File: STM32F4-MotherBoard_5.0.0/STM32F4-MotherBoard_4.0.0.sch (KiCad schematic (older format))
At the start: 1 part

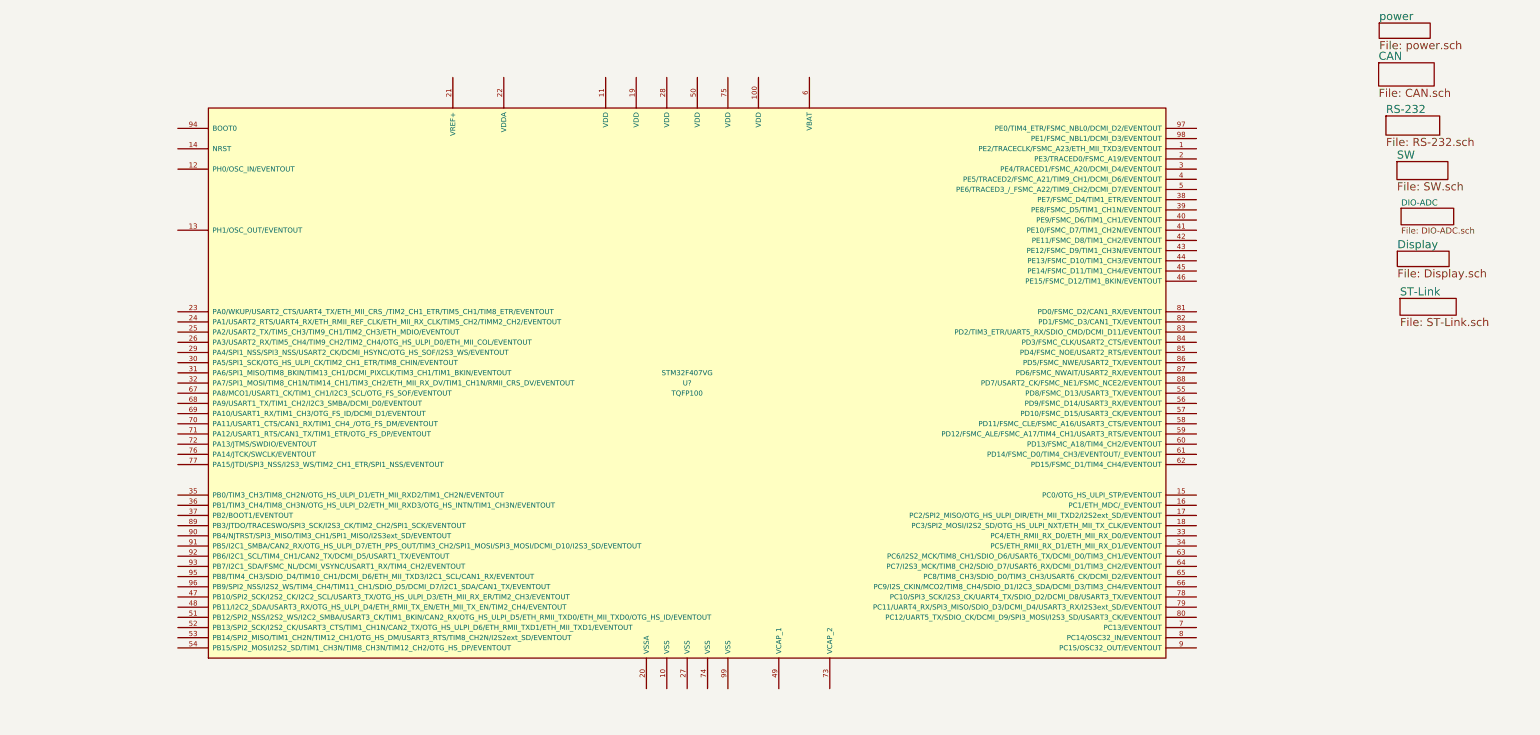
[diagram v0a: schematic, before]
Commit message: シート追加
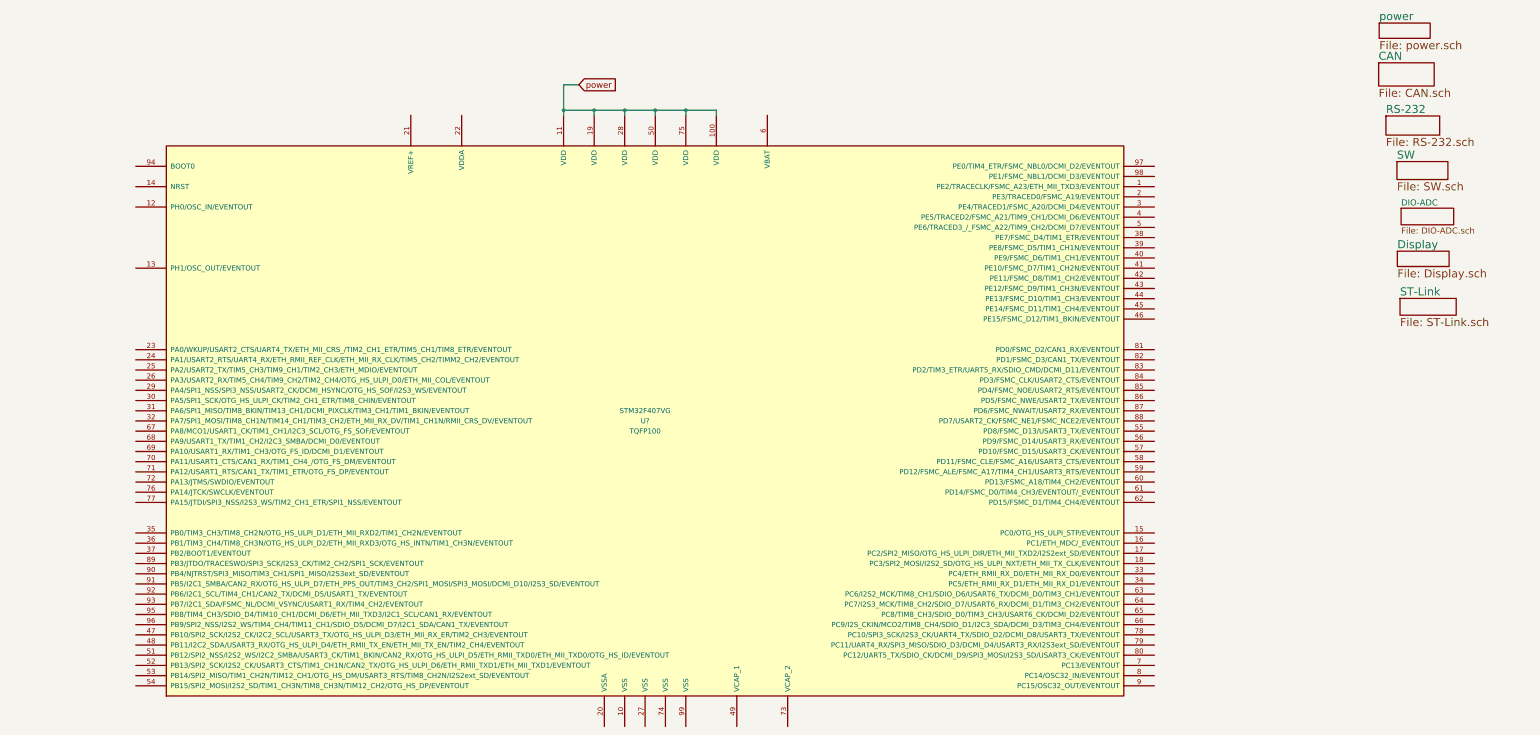
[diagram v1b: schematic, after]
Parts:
- removed U?: STM32F407VG, TQFP100, symbol STM32F407VG
- added U?: STM32F407VG, TQFP100, symbol STM32F407VG
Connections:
- new net power: U?.100 (VDD), U?.11 (VDD), U?.19 (VDD), U?.28 (VDD), U?.50 (VDD), U?.75 (VDD)
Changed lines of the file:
@@
 Comment4 ""
 $EndDescr
-$Comp
-L STM32F407VG U?
-U 1 1 589AA55C
-P 8063 5478
-F 0 "U?" H 8063 5478 50  0000 C CNN
-F 1 "STM32F407VG" H 8063 5578 50  0000 C CNN
-F 2 "TQFP100" H 8063 5378 50  0000 C CNN
-F 3 "" H 8063 5478 50  0000 C CNN
-	1    8063 5478
-	1    0    0    -1
-$EndComp
 $Sheet
 S 14857 1944 500  150
@@
 F1 "ST-Link.sch" 79
 $EndSheet
+$Comp
+L STM32F407VG U?
+U 1 1 589AAFA6
+P 7650 5850
+F 0 "U?" H 7650 5850 50  0000 C CNN
+F 1 "STM32F407VG" H 7650 5950 50  0000 C CNN
+F 2 "TQFP100" H 7650 5750 50  0000 C CNN
+F 3 "" H 7650 5850 50  0000 C CNN
+	1    7650 5850
+	1    0    0    -1
+$EndComp
+Wire Wire Line
+	8350 2850 8350 2800
+Wire Wire Line
+	8350 2800 6850 2800
+Wire Wire Line
+	6850 2550 6850 2850
+Wire Wire Line
+	7150 2850 7150 2800
+Connection ~ 7150 2800
+Wire Wire Line
+	7450 2850 7450 2800
+Connection ~ 7450 2800
+Wire Wire Line
+	7750 2850 7750 2800
+Connection ~ 7750 2800
+Wire Wire Line
+	8050 2850 8050 2800
+Connection ~ 8050 2800
+Wire Wire Line
+	6850 2550 7000 2550
+Connection ~ 6850 2800
+Text GLabel 7000 2550 2    60   Input ~ 0
+power
 $EndSCHEMATC

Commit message: ラベルの作成
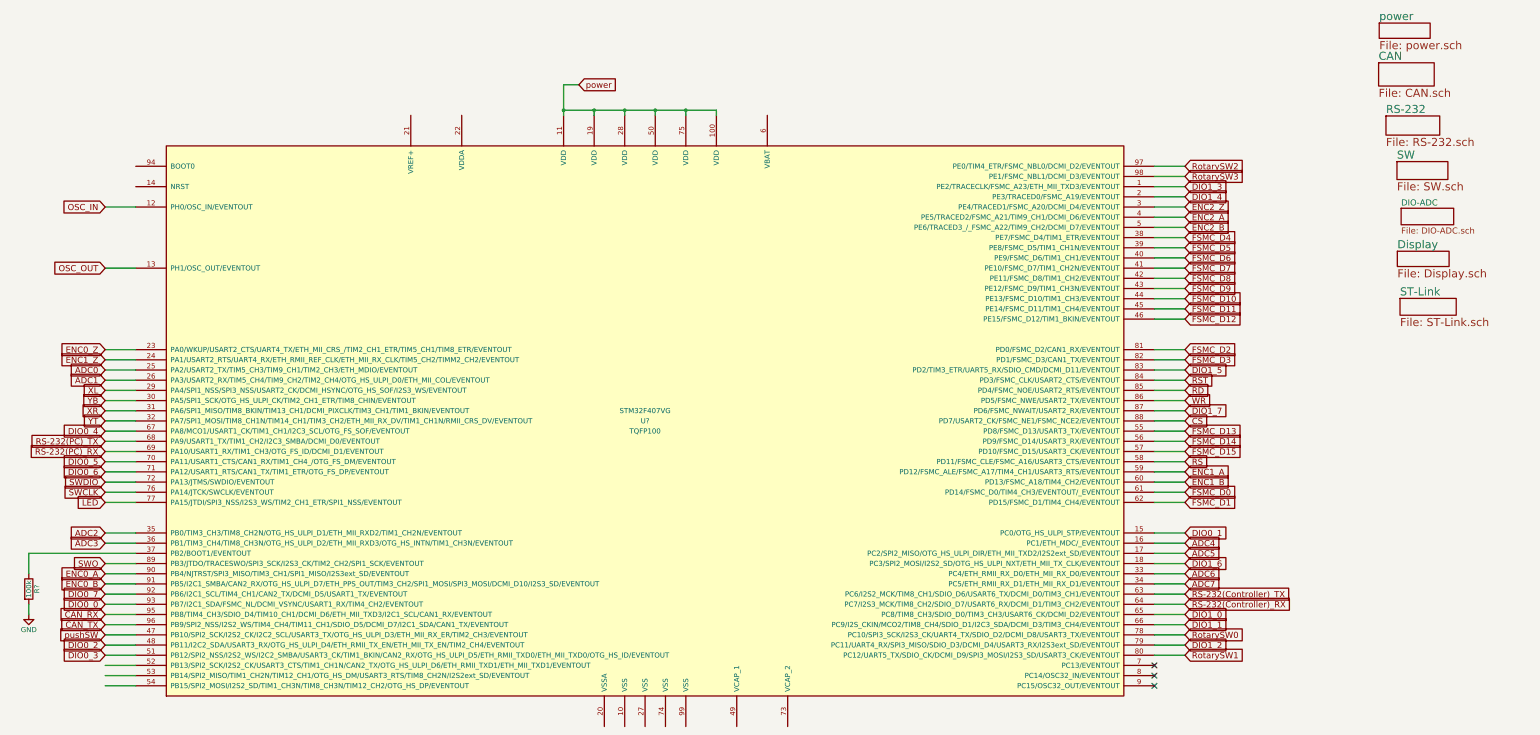
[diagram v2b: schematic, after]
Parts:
- added R?: 100k, symbol R
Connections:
- net DIO1_3: now reaches U?.1 (PE2/TRACECLK/FSMC_A23/ETH_MII_TXD3/EVENTOUT)
- net OSC_IN: now reaches U?.12 (PH0/OSC_IN/EVENTOUT)
- net OSC_OUT: now reaches U?.13 (PH1/OSC_OUT/EVENTOUT)
- net DIO0_1: now reaches U?.15 (PC0/OTG_HS_ULPI_STP/EVENTOUT)
- net ADC4: now reaches U?.16 (PC1/ETH_MDC/_EVENTOUT)
- net ADC5: now reaches U?.17 (PC2/SPI2_MISO/OTG_HS_ULPI_DIR/ETH_MII_TXD2/I2S2ext_SD/EVENTOUT)
- net DIO1_6: now reaches U?.18 (PC3/SPI2_MOSI/I2S2_SD/OTG_HS_ULPI_NXT/ETH_MII_TX_CLK/EVENTOUT)
- net DIO1_4: now reaches U?.2 (PE3/TRACED0/FSMC_A19/EVENTOUT)
- net ENC0_Z: now reaches U?.23 (PA0/WKUP/USART2_CTS/UART4_TX/ETH_MII_CRS_/TIM2_CH1_ETR/TIM5_CH1/TIM8_ETR/EVENTOUT)
- net ENC1_Z: now reaches U?.24 (PA1/USART2_RTS/UART4_RX/ETH_RMII_REF_CLK/ETH_MII_RX_CLK/TIM5_CH2/TIMM2_CH2/EVENTOUT)
- net ADC0: now reaches U?.25 (PA2/USART2_TX/TIM5_CH3/TIM9_CH1/TIM2_CH3/ETH_MDIO/EVENTOUT)
- net ADC1: now reaches U?.26 (PA3/USART2_RX/TIM5_CH4/TIM9_CH2/TIM2_CH4/OTG_HS_ULPI_D0/ETH_MII_COL/EVENTOUT)
- net XL: now reaches U?.29 (PA4/SPI1_NSS/SPI3_NSS/USART2_CK/DCMI_HSYNC/OTG_HS_SOF/I2S3_WS/EVENTOUT)
- net ENC2_Z: now reaches U?.3 (PE4/TRACED1/FSMC_A20/DCMI_D4/EVENTOUT)
- net YB: now reaches U?.30 (PA5/SPI1_SCK/OTG_HS_ULPI_CK/TIM2_CH1_ETR/TIM8_CHIN/EVENTOUT)
- net XR: now reaches U?.31 (PA6/SPI1_MISO/TIM8_BKIN/TIM13_CH1/DCMI_PIXCLK/TIM3_CH1/TIM1_BKIN/EVENTOUT)
- net YT: now reaches U?.32 (PA7/SPI1_MOSI/TIM8_CH1N/TIM14_CH1/TIM3_CH2/ETH_MII_RX_DV/TIM1_CH1N/RMII_CRS_DV/EVENTOUT)
- net ADC6: now reaches U?.33 (PC4/ETH_RMII_RX_D0/ETH_MII_RX_D0/EVENTOUT)
- net ADC7: now reaches U?.34 (PC5/ETH_RMII_RX_D1/ETH_MII_RX_D1/EVENTOUT)
- net ADC2: now reaches U?.35 (PB0/TIM3_CH3/TIM8_CH2N/OTG_HS_ULPI_D1/ETH_MII_RXD2/TIM1_CH2N/EVENTOUT)
- net ADC3: now reaches U?.36 (PB1/TIM3_CH4/TIM8_CH3N/OTG_HS_ULPI_D2/ETH_MII_RXD3/OTG_HS_INTN/TIM1_CH3N/EVENTOUT)
- net at U?.37 (PB2/BOOT1/EVENTOUT): now also R?.1
- net FSMC_D4: now reaches U?.38 (PE7/FSMC_D4/TIM1_ETR/EVENTOUT)
- net FSMC_D5: now reaches U?.39 (PE8/FSMC_D5/TIM1_CH1N/EVENTOUT)
- net ENC2_A: now reaches U?.4 (PE5/TRACED2/FSMC_A21/TIM9_CH1/DCMI_D6/EVENTOUT)
- net FSMC_D6: now reaches U?.40 (PE9/FSMC_D6/TIM1_CH1/EVENTOUT)
- net FSMC_D7: now reaches U?.41 (PE10/FSMC_D7/TIM1_CH2N/EVENTOUT)
- net FSMC_D8: now reaches U?.42 (PE11/FSMC_D8/TIM1_CH2/EVENTOUT)
- net FSMC_D9: now reaches U?.43 (PE12/FSMC_D9/TIM1_CH3N/EVENTOUT)
- net FSMC_D10: now reaches U?.44 (PE13/FSMC_D10/TIM1_CH3/EVENTOUT)
- net FSMC_D11: now reaches U?.45 (PE14/FSMC_D11/TIM1_CH4/EVENTOUT)
- net FSMC_D12: now reaches U?.46 (PE15/FSMC_D12/TIM1_BKIN/EVENTOUT)
- net pushSW: now reaches U?.47 (PB10/SPI2_SCK/I2S2_CK/I2C2_SCL/USART3_TX/OTG_HS_ULPI_D3/ETH_MII_RX_ER/TIM2_CH3/EVENTOUT)
- net DIO0_2: now reaches U?.48 (PB11/I2C2_SDA/USART3_RX/OTG_HS_ULPI_D4/ETH_RMII_TX_EN/ETH_MII_TX_EN/TIM2_CH4/EVENTOUT)
- net ENC2_B: now reaches U?.5 (PE6/TRACED3_/_FSMC_A22/TIM9_CH2/DCMI_D7/EVENTOUT)
- net DIO0_3: now reaches U?.51 (PB12/SPI2_NSS/I2S2_WS/I2C2_SMBA/USART3_CK/TIM1_BKIN/CAN2_RX/OTG_HS_ULPI_D5/ETH_RMII_TXD0/ETH_MII_TXD0/OTG_HS_ID/EVENTOUT)
- net FSMC_D13: now reaches U?.55 (PD8/FSMC_D13/USART3_TX/EVENTOUT)
- net FSMC_D14: now reaches U?.56 (PD9/FSMC_D14/USART3_RX/EVENTOUT)
- net FSMC_D15: now reaches U?.57 (PD10/FSMC_D15/USART3_CK/EVENTOUT)
- net RS: now reaches U?.58 (PD11/FSMC_CLE/FSMC_A16/USART3_CTS/EVENTOUT)
- net ENC1_A: now reaches U?.59 (PD12/FSMC_ALE/FSMC_A17/TIM4_CH1/USART3_RTS/EVENTOUT)
- net ENC1_B: now reaches U?.60 (PD13/FSMC_A18/TIM4_CH2/EVENTOUT)
- net FSMC_D0: now reaches U?.61 (PD14/FSMC_D0/TIM4_CH3/EVENTOUT/_EVENTOUT)
- net FSMC_D1: now reaches U?.62 (PD15/FSMC_D1/TIM4_CH4/EVENTOUT)
- net RS-232(Controller)_TX: now reaches U?.63 (PC6/I2S2_MCK/TIM8_CH1/SDIO_D6/USART6_TX/DCMI_D0/TIM3_CH1/EVENTOUT)
- net RS-232(Controller)_RX: now reaches U?.64 (PC7/I2S3_MCK/TIM8_CH2/SDIO_D7/USART6_RX/DCMI_D1/TIM3_CH2/EVENTOUT)
- net DIO1_0: now reaches U?.65 (PC8/TIM8_CH3/SDIO_D0/TIM3_CH3/USART6_CK/DCMI_D2/EVENTOUT)
- net DIO1_1: now reaches U?.66 (PC9/I2S_CKIN/MCO2/TIM8_CH4/SDIO_D1/I2C3_SDA/DCMI_D3/TIM3_CH4/EVENTOUT)
- net DIO0_4: now reaches U?.67 (PA8/MCO1/USART1_CK/TIM1_CH1/I2C3_SCL/OTG_FS_SOF/EVENTOUT)
- net RS-232(PC)_TX: now reaches U?.68 (PA9/USART1_TX/TIM1_CH2/I2C3_SMBA/DCMI_D0/EVENTOUT)
- net RS-232(PC)_RX: now reaches U?.69 (PA10/USART1_RX/TIM1_CH3/OTG_FS_ID/DCMI_D1/EVENTOUT)
- net DIO0_5: now reaches U?.70 (PA11/USART1_CTS/CAN1_RX/TIM1_CH4_/OTG_FS_DM/EVENTOUT)
- net DIO0_6: now reaches U?.71 (PA12/USART1_RTS/CAN1_TX/TIM1_ETR/OTG_FS_DP/EVENTOUT)
- net SWDIO: now reaches U?.72 (PA13/JTMS/SWDIO/EVENTOUT)
- net SWCLK: now reaches U?.76 (PA14/JTCK/SWCLK/EVENTOUT)
- net LED: now reaches U?.77 (PA15/JTDI/SPI3_NSS/I2S3_WS/TIM2_CH1_ETR/SPI1_NSS/EVENTOUT)
- net RotarySW0: now reaches U?.78 (PC10/SPI3_SCK/I2S3_CK/UART4_TX/SDIO_D2/DCMI_D8/USART3_TX/EVENTOUT)
- net DIO1_2: now reaches U?.79 (PC11/UART4_RX/SPI3_MISO/SDIO_D3/DCMI_D4/USART3_RX/I2S3ext_SD/EVENTOUT)
- net RotarySW1: now reaches U?.80 (PC12/UART5_TX/SDIO_CK/DCMI_D9/SPI3_MOSI/I2S3_SD/USART3_CK/EVENTOUT)
- net FSMC_D2: now reaches U?.81 (PD0/FSMC_D2/CAN1_RX/EVENTOUT)
- net FSMC_D3: now reaches U?.82 (PD1/FSMC_D3/CAN1_TX/EVENTOUT)
- net DIO1_5: now reaches U?.83 (PD2/TIM3_ETR/UART5_RX/SDIO_CMD/DCMI_D11/EVENTOUT)
- net RST: now reaches U?.84 (PD3/FSMC_CLK/USART2_CTS/EVENTOUT)
- net RD: now reaches U?.85 (PD4/FSMC_NOE/USART2_RTS/EVENTOUT)
- net WR: now reaches U?.86 (PD5/FSMC_NWE/USART2_TX/EVENTOUT)
- net DIO1_7: now reaches U?.87 (PD6/FSMC_NWAIT/USART2_RX/EVENTOUT)
- net CS: now reaches U?.88 (PD7/USART2_CK/FSMC_NE1/FSMC_NCE2/EVENTOUT)
- net SWO: now reaches U?.89 (PB3/JTDO/TRACESWO/SPI3_SCK/I2S3_CK/TIM2_CH2/SPI1_SCK/EVENTOUT)
- net ENC0_A: now reaches U?.90 (PB4/NJTRST/SPI3_MISO/TIM3_CH1/SPI1_MISO/I2S3ext_SD/EVENTOUT)
- net ENC0_B: now reaches U?.91 (PB5/I2C1_SMBA/CAN2_RX/OTG_HS_ULPI_D7/ETH_PPS_OUT/TIM3_CH2/SPI1_MOSI/SPI3_MOSI/DCMI_D10/I2S3_SD/EVENTOUT)
- net DIO0_7: now reaches U?.92 (PB6/I2C1_SCL/TIM4_CH1/CAN2_TX/DCMI_D5/USART1_TX/EVENTOUT)
- net DIO0_0: now reaches U?.93 (PB7/I2C1_SDA/FSMC_NL/DCMI_VSYNC/USART1_RX/TIM4_CH2/EVENTOUT)
- net CAN_RX: now reaches U?.95 (PB8/TIM4_CH3/SDIO_D4/TIM10_CH1/DCMI_D6/ETH_MII_TXD3/I2C1_SCL/CAN1_RX/EVENTOUT)
- net CAN_TX: now reaches U?.96 (PB9/SPI2_NSS/I2S2_WS/TIM4_CH4/TIM11_CH1/SDIO_D5/DCMI_D7/I2C1_SDA/CAN1_TX/EVENTOUT)
- net RotarySW2: now reaches U?.97 (PE0/TIM4_ETR/FSMC_NBL0/DCMI_D2/EVENTOUT)
- net RotarySW3: now reaches U?.98 (PE1/FSMC_NBL1/DCMI_D3/EVENTOUT)
- new net GND: R?.2
- no-connect marks 0 -> 3
